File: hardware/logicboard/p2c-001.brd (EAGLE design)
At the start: 91 x 55 mm, 51 parts, among them IC1 74LS07N, K1 G5V1, T1 2SC1815

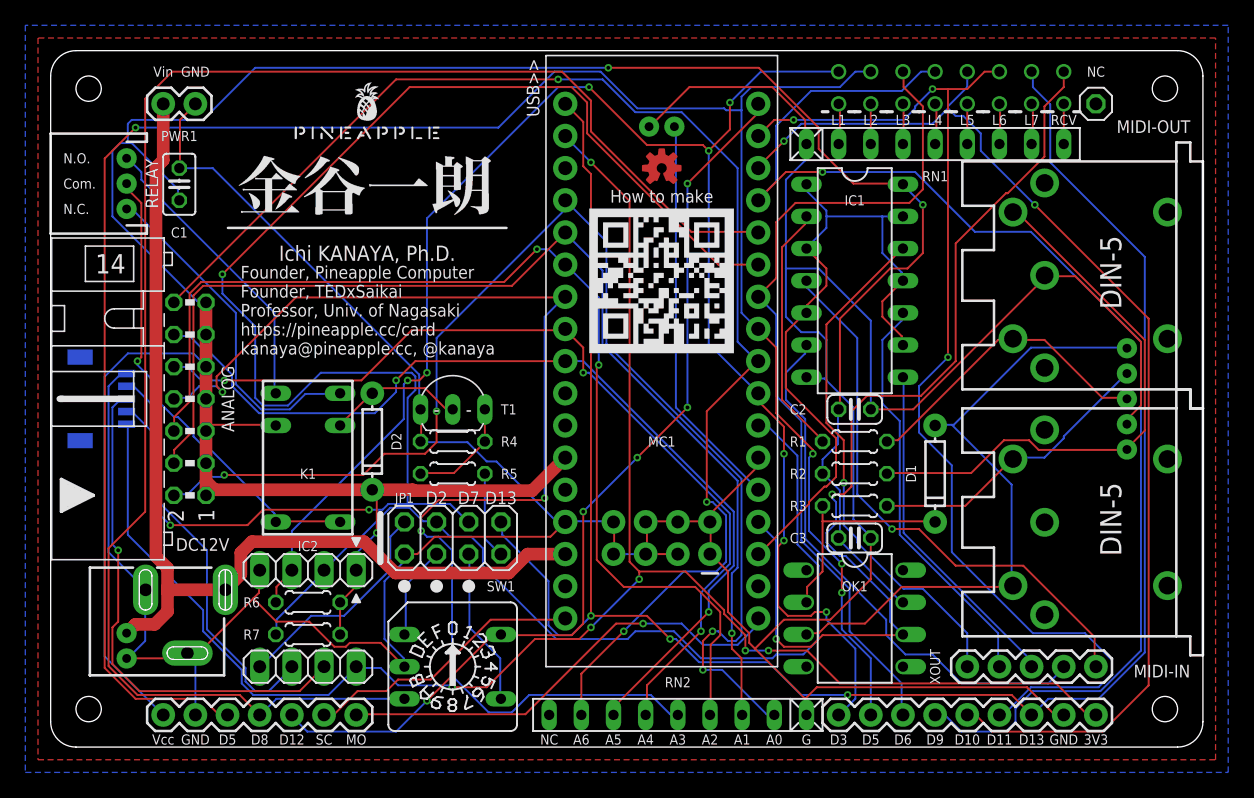
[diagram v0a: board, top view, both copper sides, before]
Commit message: Changed pattern.
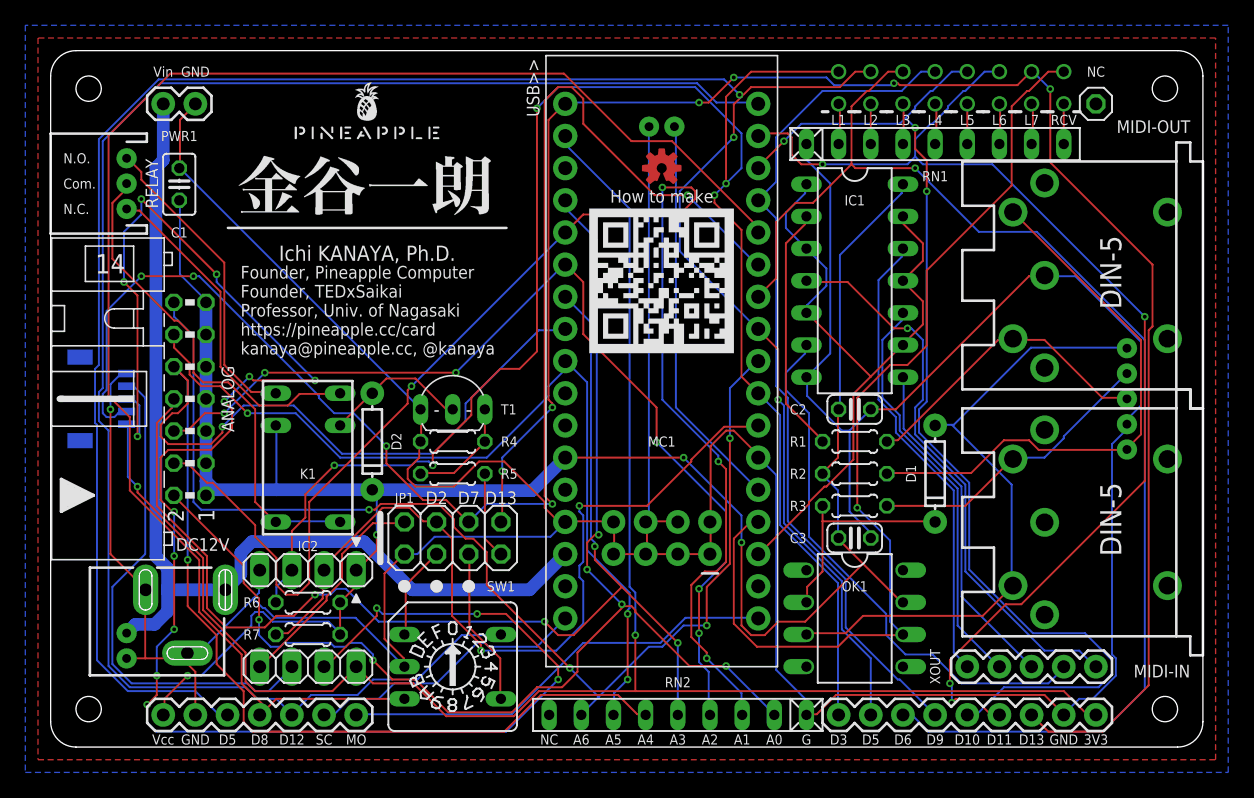
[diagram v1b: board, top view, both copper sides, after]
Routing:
- net SCL: track 40.5 -> 141.2 mm, vias 1 -> 15
- net VCC: track 235.7 -> 167.2 mm, vias 3 -> 4
- net SW_3: track 74.0 -> 131.5 mm, vias 5 -> 0
- net ANLG_4: track 71.9 -> 111.6 mm, vias 3 -> 2
- net PWM_3: track 102.0 -> 66.8 mm, vias 1 -> 0
- net PWM_2: track 66.9 -> 101.6 mm, vias 0 -> 1
- net ANLG_1: track 89.6 -> 115.0 mm, vias 1 -> 4
- net GND: track 319.3 -> 343.4 mm, vias 0 -> 1
- net PWM_6: track 154.0 -> 137.9 mm, vias 3 -> 6
- net ANLG_6: track 107.6 -> 92.5 mm, vias 3 -> 4
- net SW_1: track 126.4 -> 112.7 mm, vias 3 -> 5
- net ANLG_2: track 87.4 -> 78.5 mm, vias 2 -> 6
- net SW_0: track 74.0 -> 65.9 mm, vias 0 -> 2
- net PWM_0: track 131.1 -> 139.1 mm, vias 8 -> 5
- net SDA: track 32.4 -> 39.9 mm
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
